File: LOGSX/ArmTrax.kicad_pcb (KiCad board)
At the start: 4 copper layers, 94 parts, among them IC1 STM32G473CET6, IC2 STC3117IJT, J1 Conn_01x02, J2 BATTERY CONN, J3 POWER IN, J4 SMA_Edge, J5 SMA_Edge, SW1 SW_SPDT, U1 W25Q32JVSS, U2 LT1129-3.3_SO8, U3 MCP73113_4, U4 TESEO-LIV3F, U5 BGA725L6E6327FTSA1, U6 SX1273, U7 PE4259, U8 B4327, Y1 Crystal_GND24, Y2 Crystal_GND24, Y3 Crystal_GND24

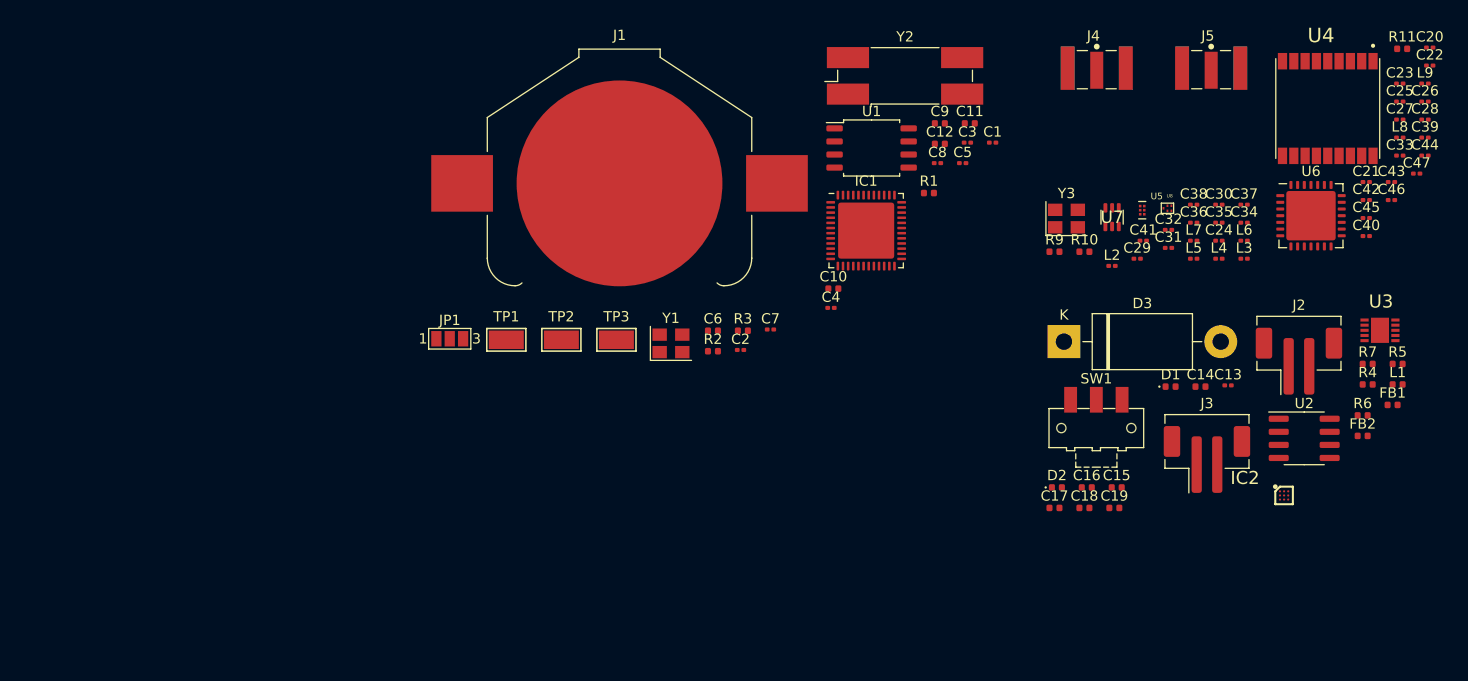
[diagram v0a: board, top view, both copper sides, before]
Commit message: Add files via upload
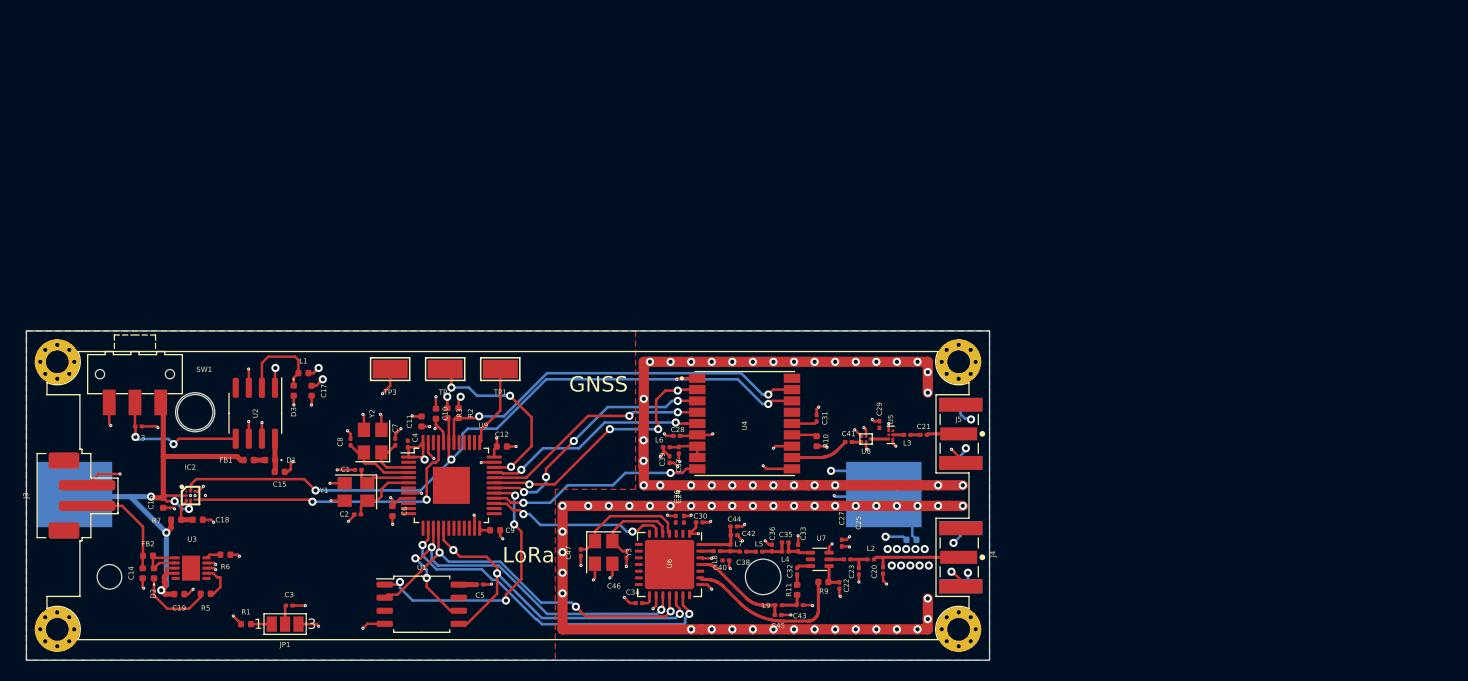
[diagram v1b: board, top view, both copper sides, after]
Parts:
- removed IC1: STM32G473CET6, Package_DFN_QFN:QFN-48-1EP_7x7mm_P0.5mm_EP5.45x5.45mm
- removed J1: Conn_01x02, Battery:BatteryHolder_Keystone_3008_1x2450
- added REF**: MountingHole_2.2mm_M2_Pad_Via, MountingHole:MountingHole_2.2mm_M2_Pad_Via, F.Cu at (150.4, 76.7)
- added REF**: MountingHole_2.2mm_M2_Pad_Via, MountingHole:MountingHole_2.2mm_M2_Pad_Via, F.Cu at (150.4, 50.7)
- added REF**: MountingHole_2.2mm_M2_Pad_Via, MountingHole:MountingHole_2.2mm_M2_Pad_Via, F.Cu at (62.8, 76.7)
- added REF**: MountingHole_2.2mm_M2_Pad_Via, MountingHole:MountingHole_2.2mm_M2_Pad_Via, F.Cu at (62.8, 50.7)
- added U9: STM32F103C8Tx, Package_QFP:LQFP-48-1EP_7x7mm_P0.5mm_EP3.6x3.6mm, F.Cu at (101.1, 62.7)
- D3: footprint Diode_THT:D_DO-201AD_P15.24mm_Horizontal -> Diode_SMD:D_0402_1005Metric
- J2: footprint Connector_JST:JST_PH_B2B-PH-SM4-TB_1x02-1MP_P2.00mm_Vertical -> Battery:BatteryHolder_Keystone_1042_1x18650; moved to B.Cu
- R4: moved to B.Cu
- Y1, Y3: value Crystal_GND24 -> Crystal_GND23
- Y2: value Crystal_GND24 -> Crystal_GND23; footprint Crystal:Crystal_SMD_SeikoEpson_MA506-4Pin_12.7x5.1mm -> Crystal:Crystal_SMD_Abracon_ABM8G-4Pin_3.2x2.5mm
- moved FB2 118.6 mm to (71.6, 69.5), turned to 180 degrees
- moved R5 118.0 mm to (77.2, 73.2)
- moved U3 117.8 mm to (75.8, 70.8)
- moved R7 116.8 mm to (74.3, 66.0)
- moved R6 111.4 mm to (79.1, 69.5), turned to 180 degrees
- moved FB1 111.3 mm to (81.4, 60.2), turned to 180 degrees
- moved J3 109.4 mm to (65.2, 63.7), turned to 90 degrees
- moved L1 106.3 mm to (86.7, 51.8)
- moved IC2 106.3 mm to (75.8, 63.7)
- moved C13 106.0 mm to (70.7, 57.0)
- moved C14 104.4 mm to (71.1, 71.2), turned to 270 degrees
- moved U2 102.0 mm to (82.0, 55.7), turned to 270 degrees
- moved SW1 93.6 mm to (70.3, 51.9), turned to 180 degrees
- moved C19 91.3 mm to (74.7, 73.3)
- moved C16 89.8 mm to (73.1, 64.4), turned to 270 degrees
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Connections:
- C28 pad 2: V_BAT -> +3V3
- C4 pad 2: V_BAT -> +3V3
- J4 pad 2_1: Net-(J4-Pad2_1) -> GND
- J4 pad 2_2: Net-(J4-Pad2_1) -> GND
- J4 pad 3_1: Net-(J4-Pad2_1) -> GND
- J4 pad 3_2: Net-(J4-Pad2_1) -> GND
- U4 pad 6: V_BAT -> +3V3
- Y1 pad 3: OSC_OUT -> GND
- Y1 pad 4: GND -> OSC_OUT
- Y2 pad 3: OSC32_OUT -> GND
- Y2 pad 4: GND -> OSC32_OUT
- Y3 pad 3: XTB -> GND
- Y3 pad 4: GND -> XTB
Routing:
- net GND: track 0.00 -> 179.6 mm, vias 0 -> 123
- net Net-(IC2-PadB3): track 0.00 -> 170.0 mm, vias 0 -> 42
- net SDA: track 0.00 -> 70.4 mm, vias 0 -> 3
- net SCL: track 0.00 -> 69.6 mm, vias 0 -> 3
- net BATTERY: track 0.00 -> 55.1 mm, vias 0 -> 5
- net SCK: track 0.00 -> 38.6 mm, vias 0 -> 4
- net MOSI: track 0.00 -> 36.6 mm, vias 0 -> 3
- net MISO: track 0.00 -> 36.4 mm, vias 0 -> 3
- net +3V3: track 0.00 -> 35.9 mm, vias 0 -> 16
- net LoRa_NSS: track 0.00 -> 34.3 mm, vias 0 -> 2
- net ALM: track 0.00 -> 28.9 mm, vias 0 -> 2
- net FLASH_NSS: track 0.00 -> 26.2 mm, vias 0 -> 4
- net TX: track 0.00 -> 25.6 mm, vias 0 -> 4
- net RX: track 0.00 -> 24.4 mm, vias 0 -> 4
- net 1PPS: track 0.00 -> 22.4 mm, vias 0 -> 2
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- added copper zone on PWR, net +3V3
- added copper zone on B.Cu, net GND
- added copper zone on F.Cu, net GND
- added copper zone on GND, net GND
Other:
- board outline added: 93.6 x 32 mm
- net class Default: clearance 0.2 -> 0.12
- rule trace_clearance: 0.2 -> 0.12
- rule trace_min: 0.2 -> 0.12
- board text added: "GNSS"
- board text added: "LoRa"

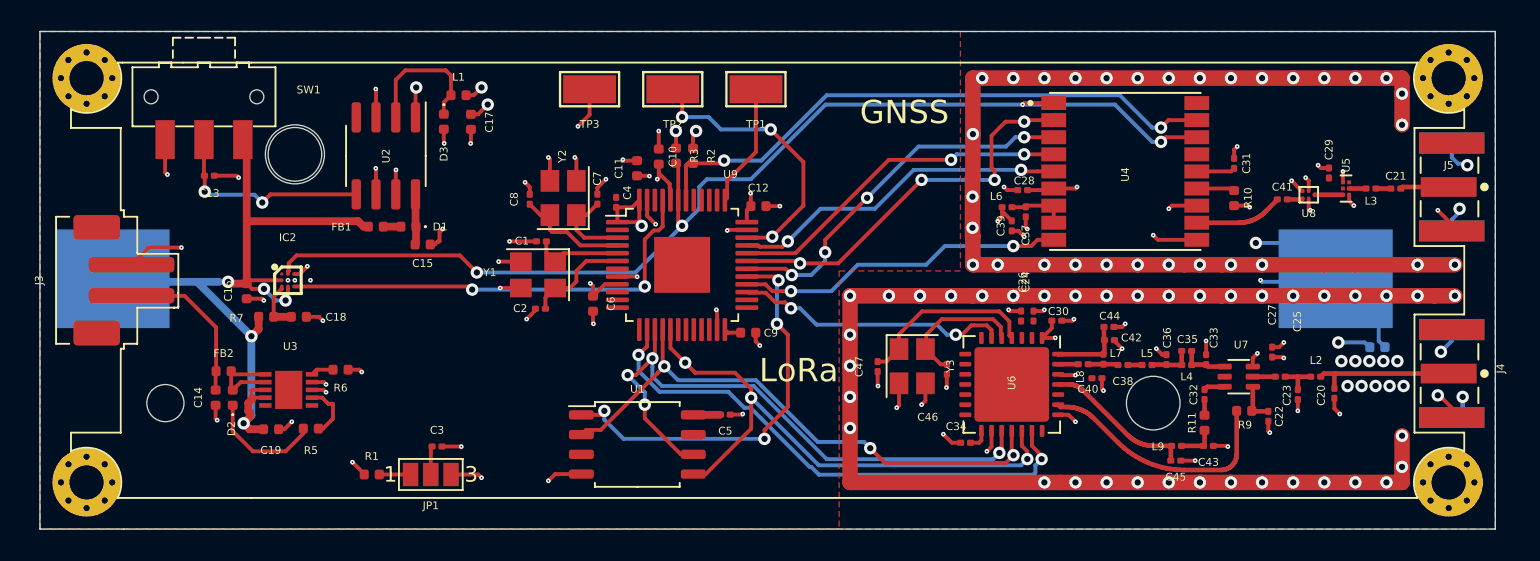
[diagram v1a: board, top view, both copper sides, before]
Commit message: Add files via upload
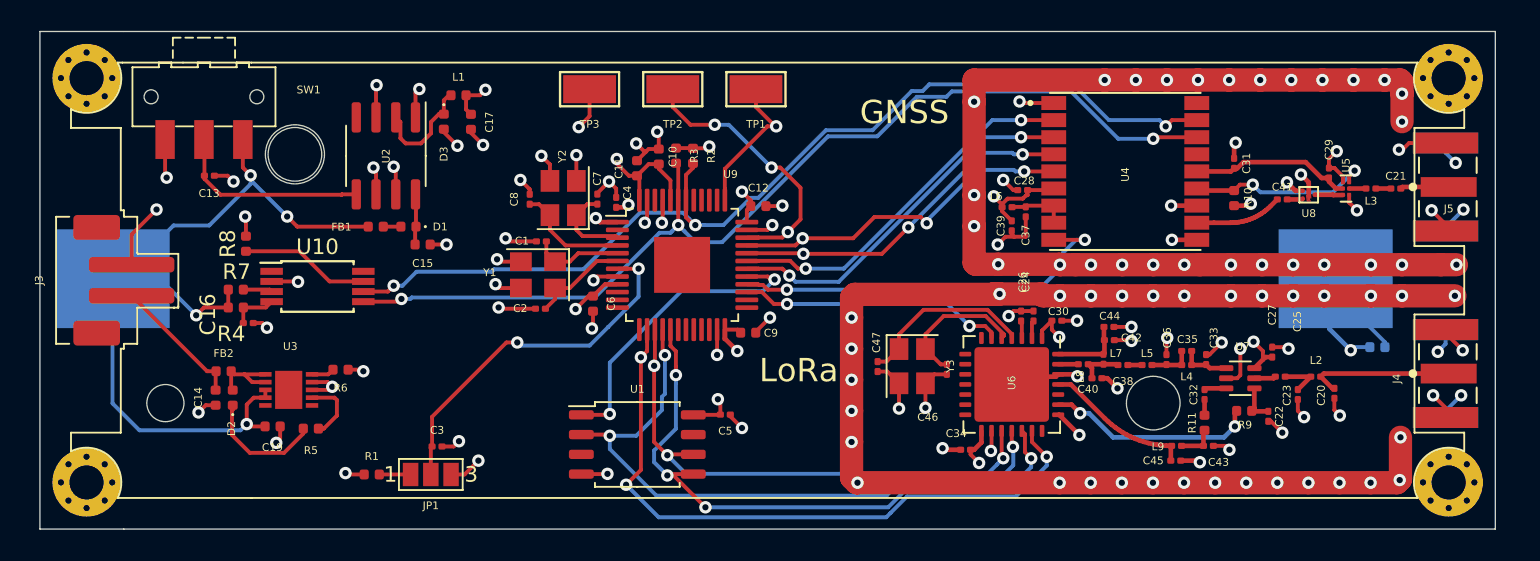
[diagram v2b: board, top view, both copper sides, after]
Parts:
- removed C18: 220nF, Capacitor_SMD:C_0402_1005Metric
- removed IC2: STC3117IJT, ASSETS:BGA9C40P3X3_146X156X66
- added R4: 500, Resistor_SMD:R_0402_1005Metric, F.Cu at (72.4, 65.5)
- added R8: 1K, Resistor_SMD:R_0402_1005Metric, F.Cu at (73.0, 61.4)
- added U10: DS2782, Package_SO:TSSOP-8_4.4x3mm_P0.65mm, F.Cu at (77.7, 64.1)
- C16: value 1uF -> 1nF; footprint Capacitor_SMD:C_0402_1005Metric -> Capacitor_SMD:C_0201_0603Metric
- moved R7 2.62 mm to (72.4, 64.3), turned to 180 degrees
- moved C16 2.05 mm to (73.2, 66.5), turned to 0 degrees
- moved C34 0.45 mm to (119.3, 74.6)
- moved C19 0.21 mm to (74.8, 73.1)
- moved U7 0.14 mm to (137.0, 70.0)
- turned J4 to 90 degrees
- turned J5 to 90 degrees
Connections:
- C16 pad 1: BATTERY -> Net-(C16-Pad1)
- J2 pad 2: Net-(IC2-PadB3) -> GND
- R4 pad 1: Net-(IC2-PadB3) -> GND
- R7 pad 1: BATTERY -> Net-(R7-Pad1)
- R7 pad 2: Net-(C18-Pad1) -> BATTERY
- U4 pad 9: SYS_RSTN -> GND
- U9 pad 28: SYS_RSTN -> GND
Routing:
- net Net-(IC2-PadB3): track 170.0 -> 0.00 mm, vias 42 -> 0
- net GND: track 179.6 -> 334.6 mm, vias 123 -> 140
- net ALM: track 28.9 -> 1.47 mm, vias 2 -> 1
- net Net-(C3-Pad1): track 1.83 -> 23.6 mm, vias 0 -> 2
- net SYS_RSTN: track 21.3 -> 0.00 mm, vias 2 -> 0
- net ANT_OFF: track 2.45 -> 12.0 mm, vias 0 -> 2
- net SNS: track 0.00 -> 8.35 mm
- net LoRa_NSS: track 34.3 -> 42.5 mm, vias 2 -> 3
- net +3V3: track 35.9 -> 44.0 mm, vias 16 -> 15
- net VCC_RF: track 2.48 -> 10.5 mm
- net FLASH_NSS: track 26.2 -> 19.8 mm, vias 4 -> 2
- net MISO: track 36.4 -> 42.3 mm
- net SDA: track 70.4 -> 65.5 mm
- net SCK: track 38.6 -> 34.5 mm, vias 4 -> 3
- net SCL: track 69.6 -> 65.5 mm
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- removed copper zone on B.Cu, net GND
